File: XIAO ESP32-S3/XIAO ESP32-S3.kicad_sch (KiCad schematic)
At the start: 6 parts, among them J1 Conn_01x07_Socket, J2 Conn_01x07_Socket, J3 Conn_01x07_Socket, J4 Conn_01x07_Socket

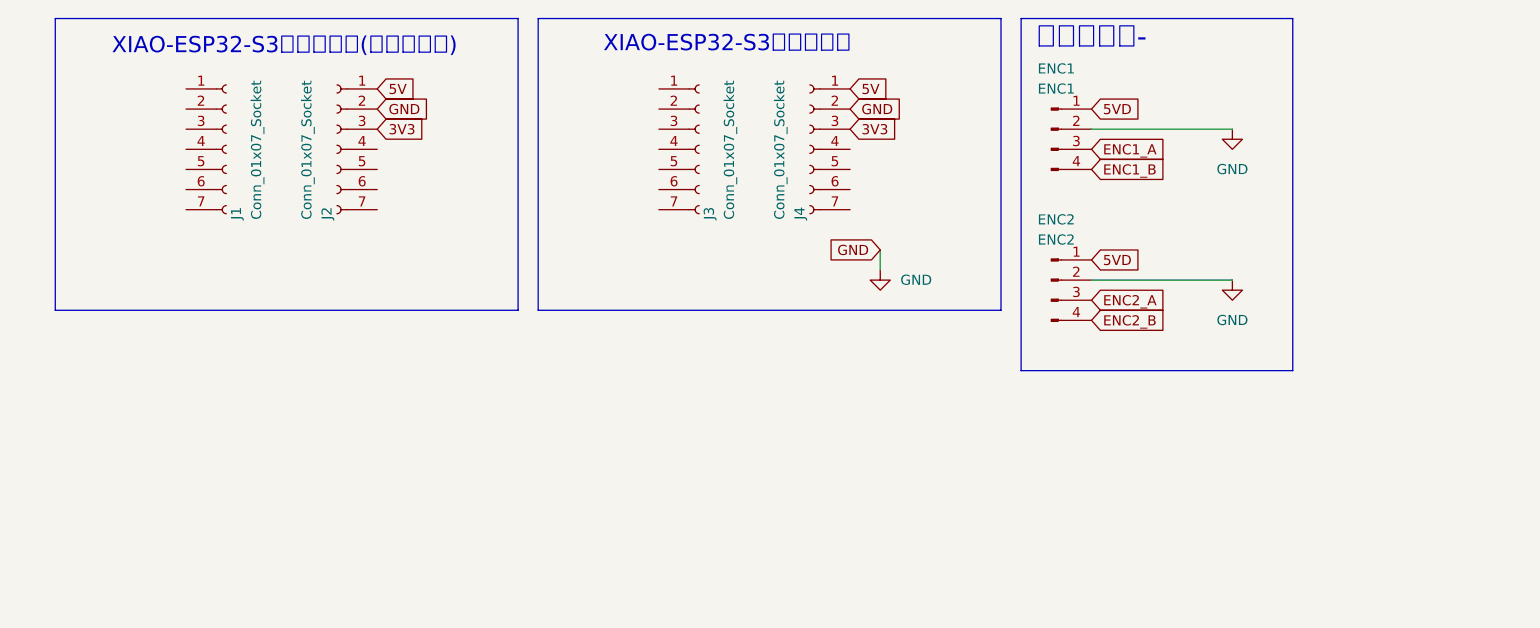
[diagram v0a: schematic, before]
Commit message: 変換基板、XIAOの回路図途中
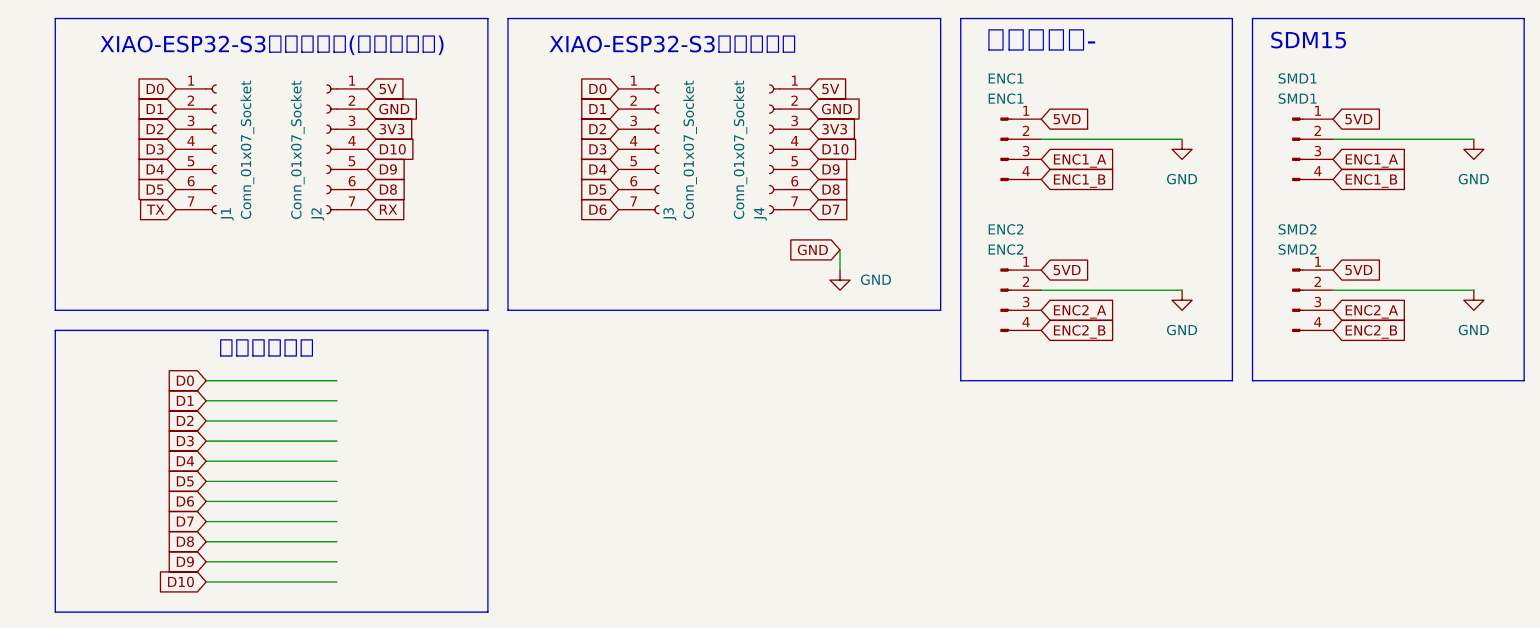
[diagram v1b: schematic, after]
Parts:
- added SMD1: SMD1, Connector_JST:JST_XH_B4B-XH-A_1x04_P2.50mm_Vertical, symbol Connector:Conn_01x04_Pin
- added SMD2: SMD2, Connector_JST:JST_XH_B4B-XH-A_1x04_P2.50mm_Vertical, symbol Connector:Conn_01x04_Pin
- J1, J2, J3, J4: footprint (none) -> Connector_PinSocket_2.54mm:PinSocket_1x07_P2.54mm_Vertical
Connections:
- net 5VD: now also SMD1.1 (Pin_1), SMD2.1 (Pin_1)
- net ENC1_A: now also SMD1.3 (Pin_3)
- net ENC1_B: now also SMD1.4 (Pin_4)
- net ENC2_A: now also SMD2.3 (Pin_3)
- net ENC2_B: now also SMD2.4 (Pin_4)
- net GND: now also SMD1.2 (Pin_2), SMD2.2 (Pin_2)
- net D10: now reaches J2.4 (Pin_4)
- net D10: now also J4.4 (Pin_4)
- net D9: now reaches J2.5 (Pin_5)
- net D9: now also J4.5 (Pin_5)
- net D8: now reaches J2.6 (Pin_6)
- net D8: now also J4.6 (Pin_6)
- net RX: now reaches J2.7 (Pin_7)
- net D7: now reaches J4.7 (Pin_7)
- net D0: now reaches J3.1 (Pin_1)
- net D0: now also J1.1 (Pin_1)
- net D1: now reaches J3.2 (Pin_2)
- net D1: now also J1.2 (Pin_2)
- net D2: now reaches J3.3 (Pin_3)
- net D2: now also J1.3 (Pin_3)
- net D3: now reaches J3.4 (Pin_4)
- net D3: now also J1.4 (Pin_4)
- net D4: now reaches J3.5 (Pin_5)
- net D4: now also J1.5 (Pin_5)
- net D5: now reaches J3.6 (Pin_6)
- net D5: now also J1.6 (Pin_6)
- net D6: now reaches J3.7 (Pin_7)
- net TX: now reaches J1.7 (Pin_7)
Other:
- note added: "SDM15"
- note added: "ピン割り当て"
- moved on the sheet: ENC1, ENC2, J1, J2, J3, J4

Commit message: SMD
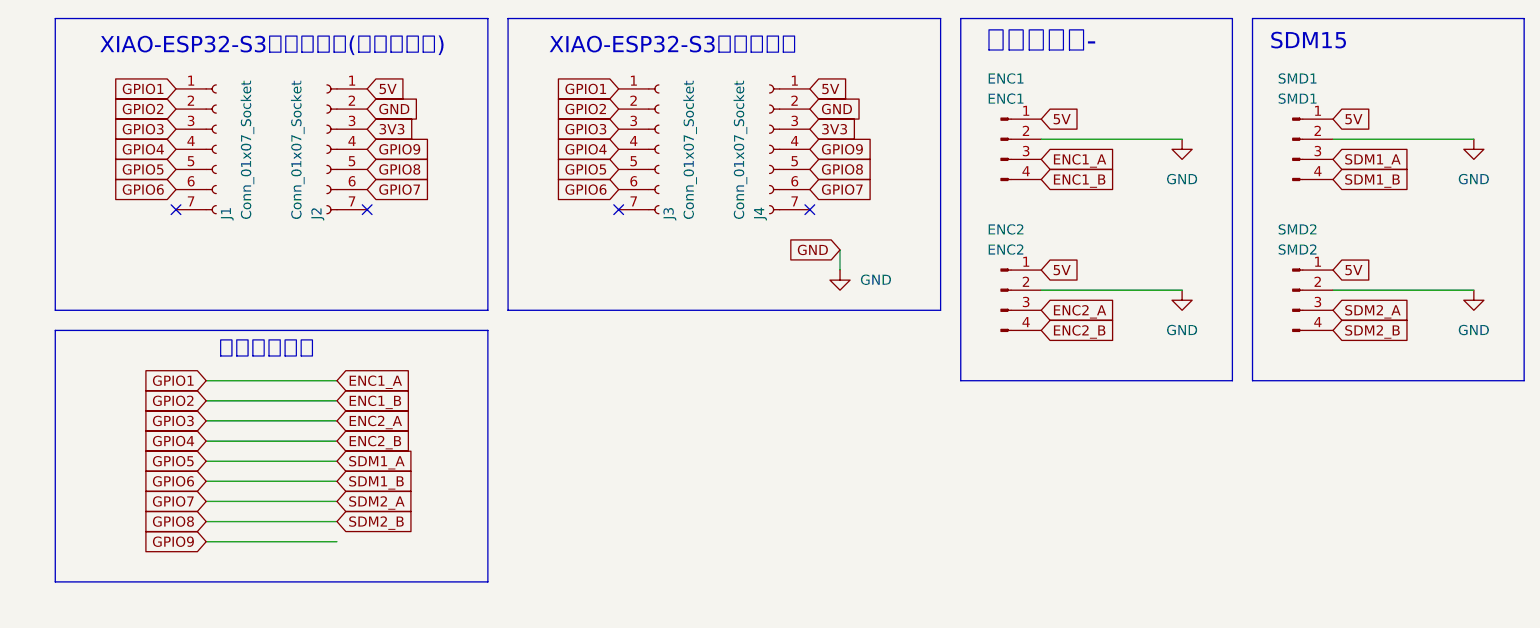
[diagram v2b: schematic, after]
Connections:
- net 5VD is gone; now on net 5V: ENC1.1 (Pin_1), ENC2.1 (Pin_1), SMD1.1 (Pin_1), SMD2.1 (Pin_1)
- net D0 is gone; now on net ENC1_A: J1.1 (Pin_1), J3.1 (Pin_1)
- net D1 is gone; now on net ENC1_B: J1.2 (Pin_2), J3.2 (Pin_2)
- net D2 is gone; now on net ENC2_A: J1.3 (Pin_3), J3.3 (Pin_3)
- net D3 is gone; now on net ENC2_B: J1.4 (Pin_4), J3.4 (Pin_4)
- net ENC1_A: no longer SMD1.3 (Pin_3)
- net ENC1_B: no longer SMD1.4 (Pin_4)
- net ENC2_A: no longer SMD2.3 (Pin_3)
- net ENC2_B: no longer SMD2.4 (Pin_4)
- net D10 renamed GPIO9
- net D4 renamed GPIO5
- net GPIO5: now also SMD1.3 (Pin_3)
- net D5 renamed GPIO6
- net GPIO6: now also SMD1.4 (Pin_4)
- net D6: no longer names the net of J3.7 (Pin_7)
- net D7: no longer names the net of J4.7 (Pin_7)
- net D8 renamed GPIO7
- net GPIO7: now also SMD2.3 (Pin_3)
- net D9 renamed GPIO8
- net GPIO8: now also SMD2.4 (Pin_4)
- net RX: no longer names the net of J2.7 (Pin_7)
- net TX: no longer names the net of J1.7 (Pin_7)
- no-connect marks 0 -> 4

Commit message: 変換基板一応できた
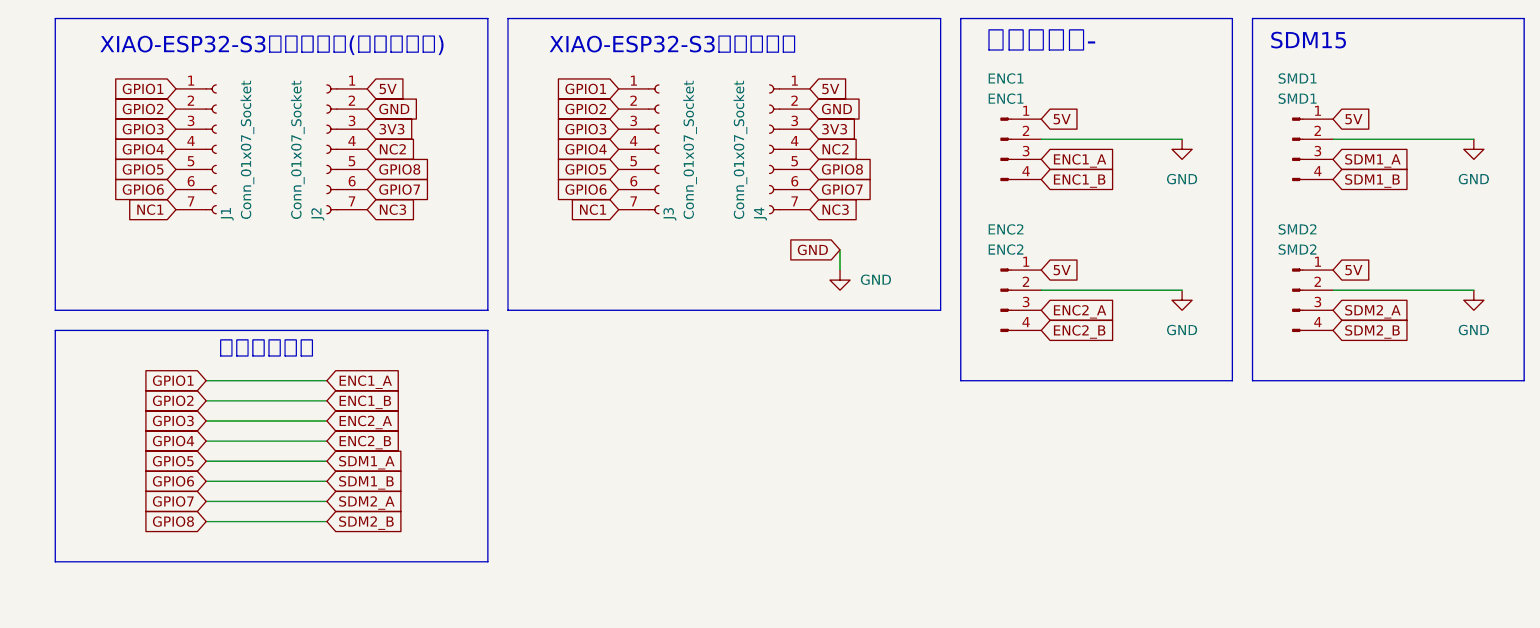
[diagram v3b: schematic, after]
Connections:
- net NC3: now reaches J2.7 (Pin_7)
- net NC3: now also J4.7 (Pin_7)
- net NC1: now reaches J3.7 (Pin_7)
- net NC1: now also J1.7 (Pin_7)
- net GPIO9 renamed NC2
- no-connect marks 4 -> 0

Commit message: 変換基板ほぼかんせ
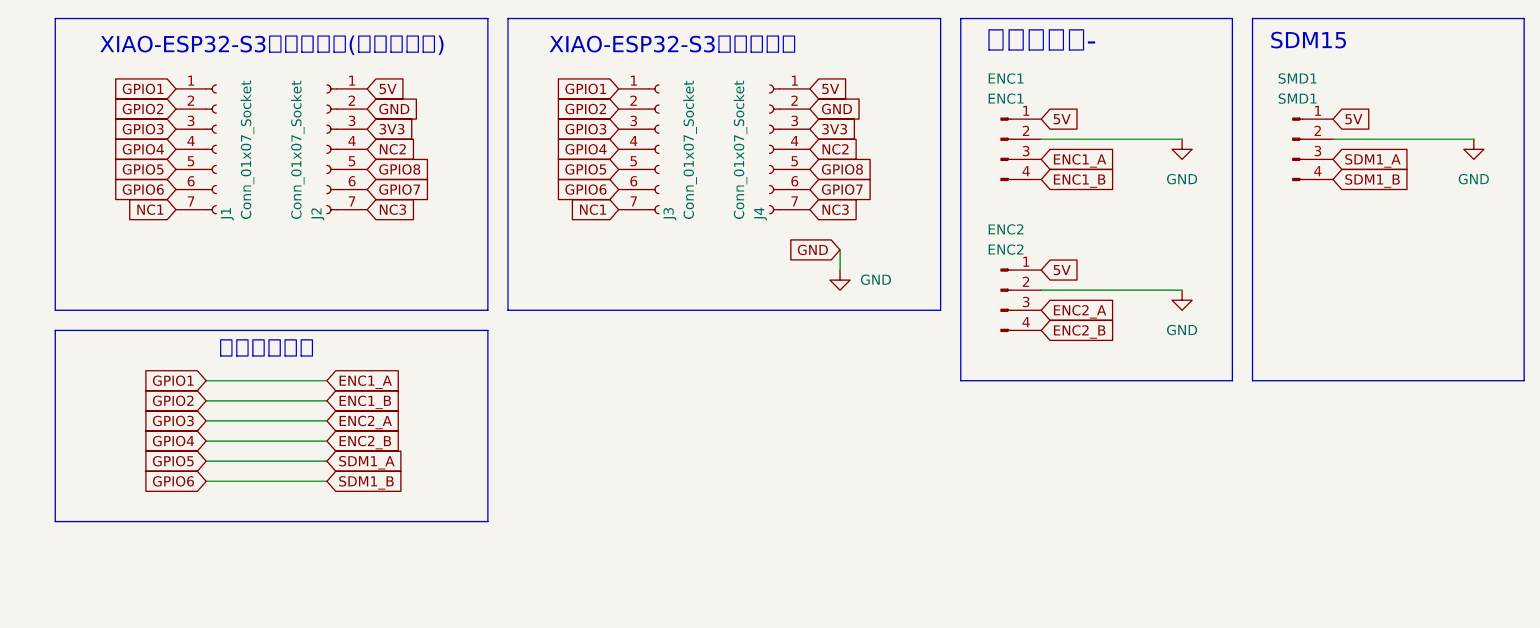
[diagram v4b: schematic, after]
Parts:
- removed SMD2: SMD2, Connector_JST:JST_XH_B4B-XH-A_1x04_P2.50mm_Vertical, symbol Connector:Conn_01x04_Pin

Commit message: 基板ほぼかんせ　ねむい
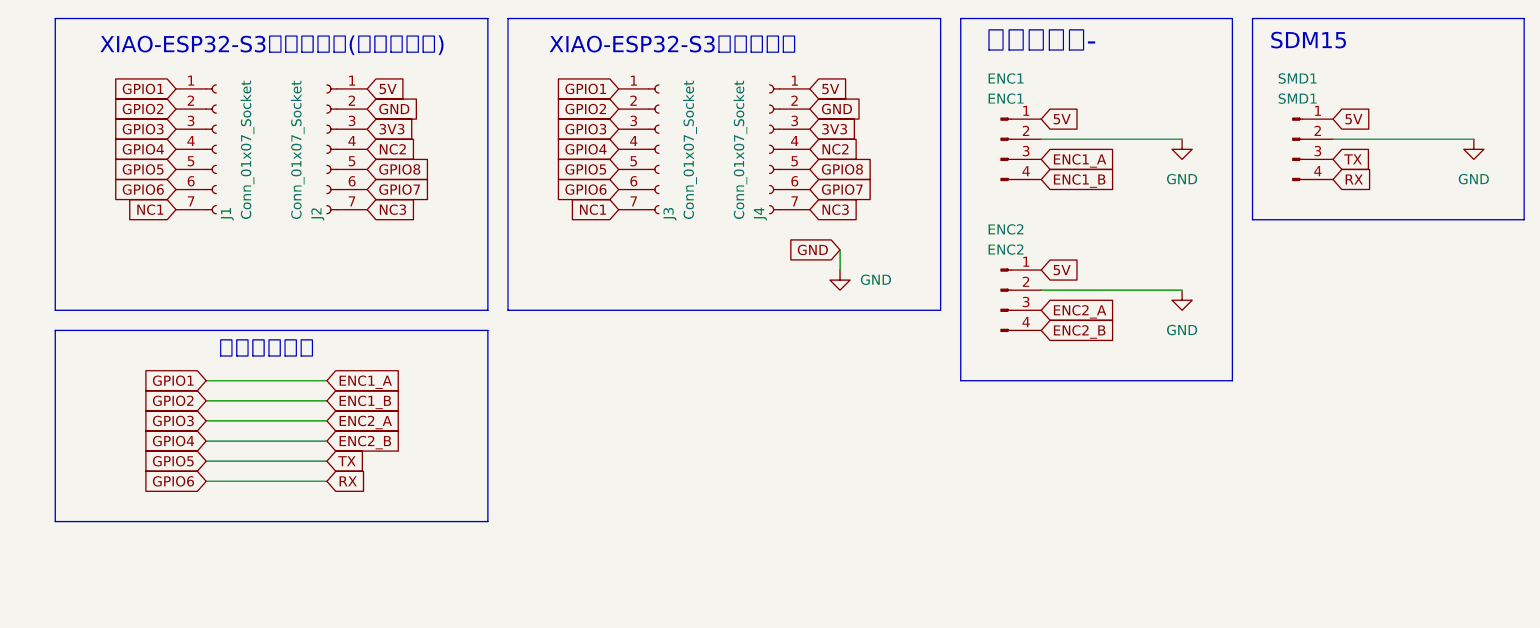
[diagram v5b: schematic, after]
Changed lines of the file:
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@@
 	(rectangle
 		(start 166.37 15.24)
-		(end 200.66 60.96)
+		(end 200.66 40.64)
 		(stroke
 			(width 0)
@@
 		)
 	)
-	(global_label "SDM1_A"
+	(global_label "TX"
 		(shape input)
 		(at 49.53 71.12 0)
@@
 		)
 		(property "Intersheetrefs" "${INTERSHEET_REFS}"
-			(at 59.7118 71.12 0)
+			(at 54.6923 71.12 0)
 			(effects
 				(font
@@
 		)
 	)
-	(global_label "SDM1_B"
+	(global_label "RX"
 		(shape input)
 		(at 49.53 73.66 0)
@@
 		)
 		(property "Intersheetrefs" "${INTERSHEET_REFS}"
-			(at 59.8932 73.66 0)
+			(at 54.9947 73.66 0)
 			(effects
 				(font
@@
 		)
 	)
-	(global_label "SDM1_A"
+	(global_label "TX"
 		(shape input)
 		(at 176.53 33.02 0)
@@
 		)
 		(property "Intersheetrefs" "${INTERSHEET_REFS}"
-			(at 186.7118 33.02 0)
-			(effects
-				(font
-					(size 1.27 1.27)
-				)
-				(justify left)
-				(hide yes)
-			)
-		)
-	)
-	(global_label "SDM1_B"
+			(at 181.6923 33.02 0)
+			(effects
+				(font
+					(size 1.27 1.27)
+				)
+				(justify left)
+				(hide yes)
+			)
+		)
+	)
+	(global_label "RX"
 		(shape input)
 		(at 176.53 35.56 0)
@@
 		)
 		(property "Intersheetrefs" "${INTERSHEET_REFS}"
-			(at 186.8932 35.56 0)
-			(effects
-				(font
+			(at 181.9947 35.56 0)
+			(effects
+				(font

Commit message: ええんちゃうの
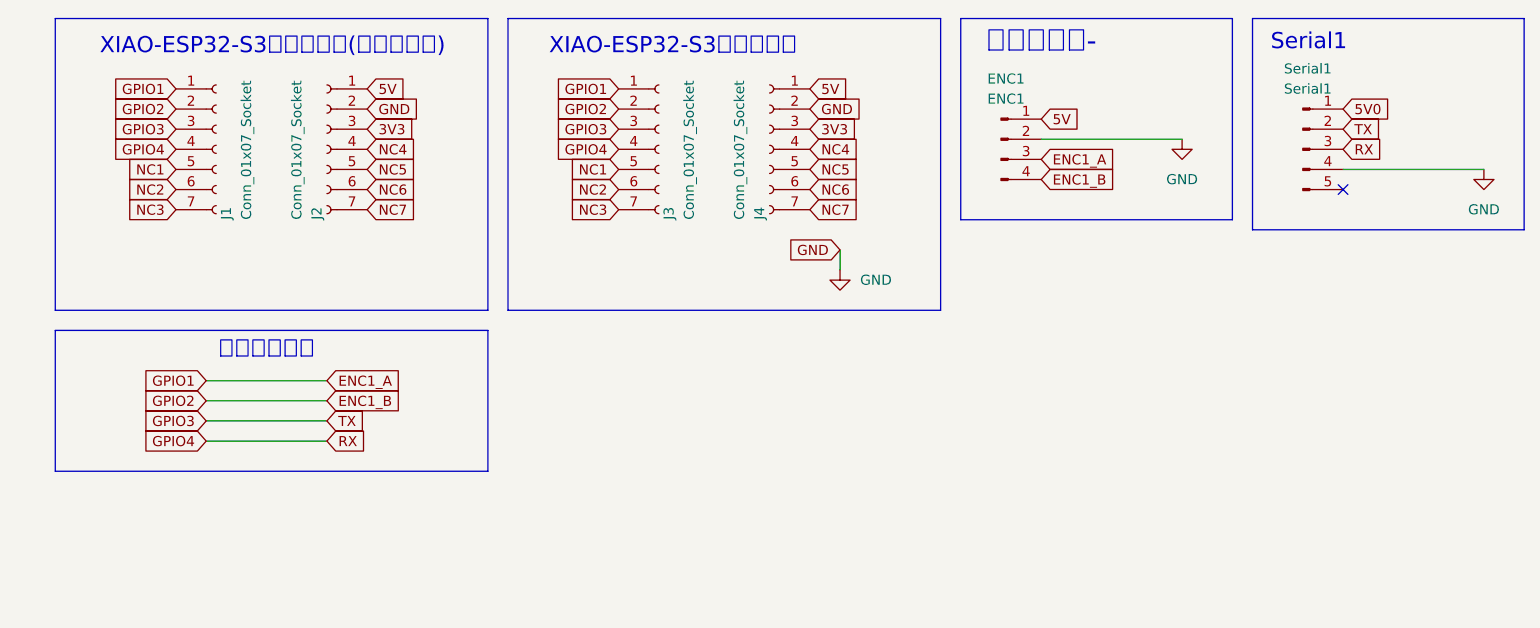
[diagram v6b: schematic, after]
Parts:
- removed ENC2: ENC2, Connector_JST:JST_XH_B4B-XH-A_1x04_P2.50mm_Vertical, symbol Connector:Conn_01x04_Pin
- removed SMD1: SMD1, Connector_JST:JST_XH_B4B-XH-A_1x04_P2.50mm_Vertical, symbol Connector:Conn_01x04_Pin
- added Serial1: Serial1, Connector_JST:JST_PH_S5B-PH-K_1x05_P2.00mm_Horizontal, symbol Connector:Conn_01x05_Pin
- ENC1: footprint Connector_JST:JST_XH_B4B-XH-A_1x04_P2.50mm_Vertical -> Connector_JST:JST_XH_S4B-XH-A_1x04_P2.50mm_Horizontal
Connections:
- net GPIO5 is gone; now on net NC1: J1.5 (Pin_5), J3.5 (Pin_5)
- net GPIO6 is gone; now on net NC2: J1.6 (Pin_6), J3.6 (Pin_6)
- net GND: now also Serial1.4 (Pin_4)
- net NC1: no longer J1.7 (Pin_7), J3.7 (Pin_7)
- net NC2: no longer J2.4 (Pin_4), J4.4 (Pin_4)
- net NC3: now also J1.7 (Pin_7), J3.7 (Pin_7); no longer J2.7 (Pin_7), J4.7 (Pin_7)
- net ENC2_A renamed GPIO3
- net GPIO3: now also Serial1.2 (Pin_2)
- net ENC2_B renamed GPIO4
- net GPIO4: now also Serial1.3 (Pin_3)
- net GPIO7 renamed NC6
- net GPIO8 renamed NC5
- new net 5V0: Serial1.1 (Pin_1)
- new net NC4: J2.4 (Pin_4), J4.4 (Pin_4)
- new net NC7: J2.7 (Pin_7), J4.7 (Pin_7)
- no-connect marks 0 -> 1
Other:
- note added: "Serial1"
- note removed: "SDM15"
